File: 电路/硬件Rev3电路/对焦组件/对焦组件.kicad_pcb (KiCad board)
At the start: 2 copper layers, 1 part, among them U1 CH32V003FxPx

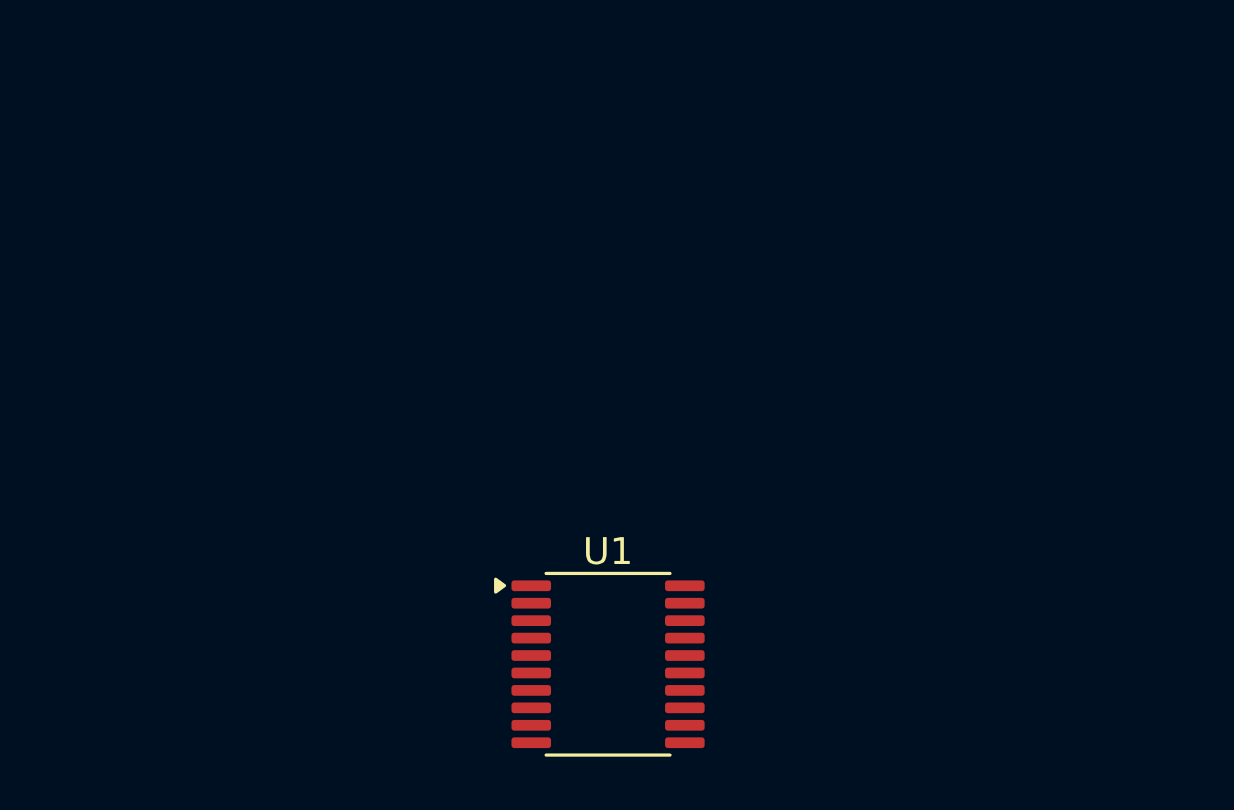
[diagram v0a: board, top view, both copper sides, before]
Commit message: 对焦驱动几乎完成
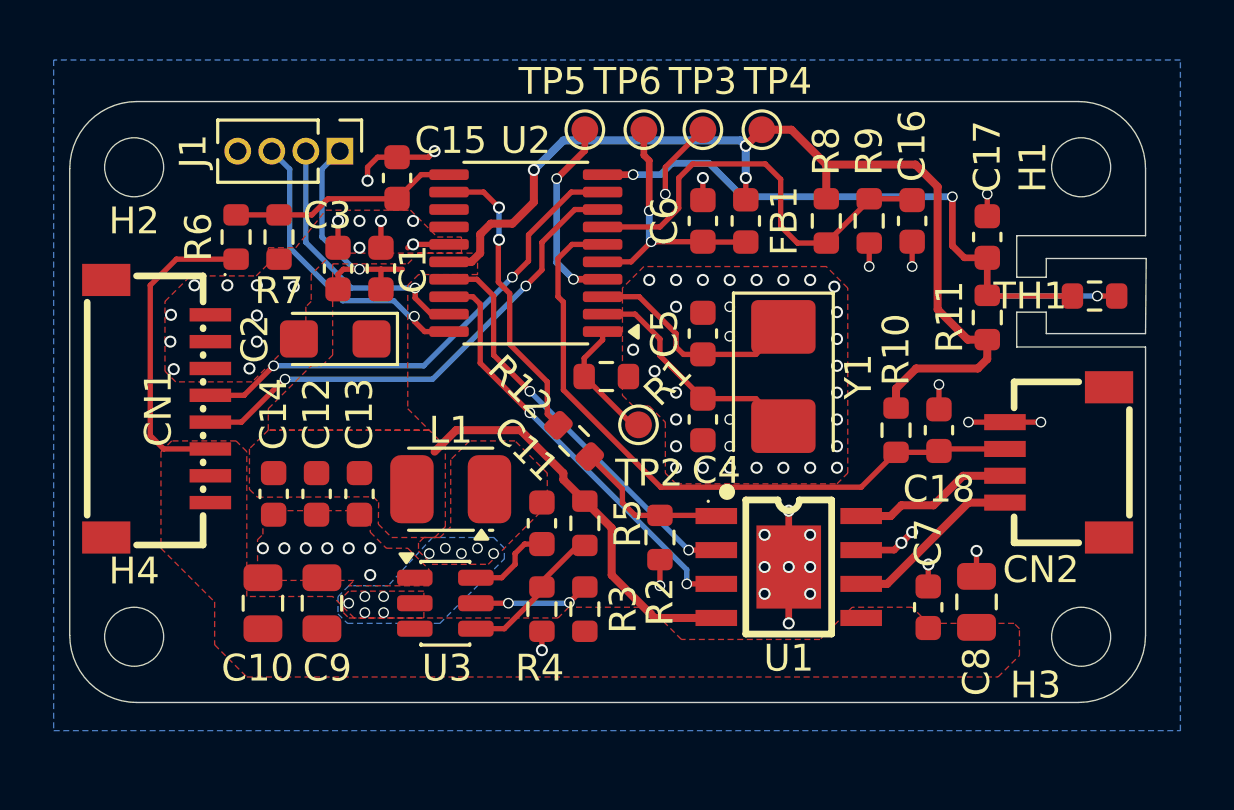
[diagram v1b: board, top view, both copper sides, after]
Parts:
- added C1: 100nf, Capacitor_SMD:C_0603_1608Metric, F.Cu at (109.3, 86.4)
- added C10: 10uf, Capacitor_SMD:C_0805_2012Metric, F.Cu at (104.9, 98.9)
- added C11: 100nf, Capacitor_SMD:C_0603_1608Metric, F.Cu at (115.3, 95.9)
- added C12: 22uf, Capacitor_SMD:C_0603_1608Metric, F.Cu at (106.9, 94.8)
- added C13: 22uf, Capacitor_SMD:C_0603_1608Metric, F.Cu at (108.5, 94.8)
- added C14: 22uf, Capacitor_SMD:C_0603_1608Metric, F.Cu at (105.3, 94.8)
- added C15: 22uf, Capacitor_SMD:C_0603_1608Metric, F.Cu at (109.9, 83.0)
- added C16: 22uf, Capacitor_SMD:C_0603_1608Metric, F.Cu at (129.1, 84.6)
- added C17: 22uf, Capacitor_SMD:C_0603_1608Metric, F.Cu at (131.9, 85.2)
- added C18: 22uf, Capacitor_SMD:C_0603_1608Metric, F.Cu at (130.1, 92.4)
- added C2: 22uf, Capacitor_Tantalum_SMD:CP_EIA-3216-18_Kemet-A, F.Cu at (107.6, 89.0)
- added C3: 1uf, Capacitor_SMD:C_0603_1608Metric, F.Cu at (107.7, 86.4)
- added C4: 20pf, Capacitor_SMD:C_0603_1608Metric, F.Cu at (121.3, 92.0)
- added C5: 20pf, Capacitor_SMD:C_0603_1608Metric, F.Cu at (121.3, 88.8)
- added C6: 100nf, Capacitor_SMD:C_0603_1608Metric, F.Cu at (121.3, 84.6)
- added C7: 100nf, Capacitor_SMD:C_0603_1608Metric, F.Cu at (129.7, 99.0)
- added C8: 47uf, Capacitor_SMD:C_0805_2012Metric, F.Cu at (131.5, 98.8)
- added C9: 10uf, Capacitor_SMD:C_0805_2012Metric, F.Cu at (107.1, 98.9)
- added CN1: HX SH-1.0-8PWT, EasyEDA:CONN-SMD_8P-P1.00_HX-SH1.0-8PWT, F.Cu at (101.0, 91.6)
- added CN2: HX SH-1.0-4PWT, EasyEDA:CONN-SMD_4P-HX-SH-1.0-4PWT, F.Cu at (134.5, 93.6)
- added FB1: FerriteBead, Inductor_SMD:L_0603_1608Metric, F.Cu at (122.9, 84.6)
- added H1: MountingHole, MountingHole:MountingHole_2.2mm_M2, F.Cu at (135.4, 82.6)
- added H2: MountingHole, MountingHole:MountingHole_2.2mm_M2, F.Cu at (100.1, 82.6)
- added H3: MountingHole, MountingHole:MountingHole_2.2mm_M2, F.Cu at (135.4, 100.1)
- added H4: MountingHole, MountingHole:MountingHole_2.2mm_M2, F.Cu at (100.1, 100.1)
- added J1: Conn_01x04_Pin, Connector_PinHeader_1.27mm:PinHeader_1x04_P1.27mm_Vertical, F.Cu at (107.8, 82.0)
- added L1: 2.2uH, Inductor_SMD:L_Coilcraft_1008HQ_2520Metric, F.Cu at (111.9, 94.6)
- added R1: 10k, Resistor_SMD:R_0603_1608Metric, F.Cu at (117.7, 90.4)
- added R10: 10k 1%, Resistor_SMD:R_0603_1608Metric, F.Cu at (128.5, 92.4)
- added R11: 10k 1%, Resistor_SMD:R_0603_1608Metric, F.Cu at (131.9, 88.2)
- added R12: 1k, Resistor_SMD:R_0603_1608Metric, F.Cu at (116.5, 92.8)
- added R2: 10k, Resistor_SMD:R_0603_1608Metric, F.Cu at (119.7, 96.4)
- added R3: 10k, Resistor_SMD:R_0603_1608Metric, F.Cu at (116.9, 99.1)
- added R4: 10k, Resistor_SMD:R_0603_1608Metric, F.Cu at (115.3, 99.1)
- added R5: 33.2k, Resistor_SMD:R_0603_1608Metric, F.Cu at (116.9, 95.9)
- added R6: 10k 1%, Resistor_SMD:R_0603_1608Metric, F.Cu at (103.9, 85.2)
- added R7: 10k 1%, Resistor_SMD:R_0603_1608Metric, F.Cu at (105.5, 85.2)
- added R8: 2.2k 1%, Resistor_SMD:R_0603_1608Metric, F.Cu at (125.9, 84.6)
- added R9: 10k 1%, Resistor_SMD:R_0603_1608Metric, F.Cu at (127.5, 84.6)
- added TH1: Thermistor_NTC, Resistor_SMD:R_0603_1608Metric, F.Cu at (135.9, 87.4)
- added TP2: BOOT, TestPoint:TestPoint_Pad_D1.0mm, F.Cu at (118.9, 92.2)
- added TP3: GND, TestPoint:TestPoint_Pad_D1.0mm, F.Cu at (121.3, 81.2)
- added TP4: 3.3V, TestPoint:TestPoint_Pad_D1.0mm, F.Cu at (123.5, 81.2)
- added TP5: NRST, TestPoint:TestPoint_Pad_D1.0mm, F.Cu at (116.9, 81.2)
- added TP6: VREF, TestPoint:TestPoint_Pad_D1.0mm, F.Cu at (119.1, 81.2)
- added U2: STM32F030F4Px, Package_SO:TSSOP-20_4.4x6.5mm_P0.65mm, F.Cu at (114.7, 85.8)
- added U3: TPS563201, Package_TO_SOT_SMD:SOT-23-6, F.Cu at (111.7, 98.9)
- added Y1: 8Mhz, Crystal:Crystal_SMD_5032-2Pin_5.0x3.2mm, F.Cu at (124.3, 90.4)
- U1: value CH32V003FxPx -> DRV8251ADDAR; footprint Package_SO:TSSOP-20_4.4x6.5mm_P0.65mm -> EasyEDA:SOPOWERPAD-8_L4.9-W3.9-P1.27-LS6.0-TL-EP
- moved U1 7.65 mm to (124.5, 97.5)
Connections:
- U1 pad 1: unconnected-(U1-PD4-Pad1) -> Net-(U1-IPROPI)
- U1 pad 2: unconnected-(U1-PD5-Pad2) -> /MotorPWM_B
- U1 pad 3: unconnected-(U1-PD6-Pad3) -> /MotorPWM_A
- U1 pad 4: unconnected-(U1-PD7-Pad4) -> +3V3
- U1 pad 5: unconnected-(U1-PA1-Pad5) -> +6V
- U1 pad 6: unconnected-(U1-PA2-Pad6) -> /MOT_A
- U1 pad 7: unconnected-(U1-VSS-Pad7) -> GND
- U1 pad 8: unconnected-(U1-PD0-Pad8) -> /MOT_B
- U1 pad 9: unconnected-(U1-VDD-Pad9) -> GND
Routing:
- net +3V3: track 0.00 -> 62.0 mm, vias 0 -> 4
- net GND: track 0.00 -> 31.5 mm, vias 0 -> 80
- net /ADC_NTC1: track 0.00 -> 25.4 mm
- net /ADC_NTC2: track 0.00 -> 21.9 mm, vias 0 -> 2
- net /USART1 _TX: track 0.00 -> 18.6 mm, vias 0 -> 2
- net /USART1 _RX: track 0.00 -> 18.4 mm, vias 0 -> 2
- net /ADC_3V3: track 0.00 -> 16.3 mm
- net /MotorPWM_A: track 0.00 -> 16.0 mm, vias 0 -> 2
- net /MotorPWM_B: track 0.00 -> 15.4 mm, vias 0 -> 2
- net +6V: track 0.00 -> 11.6 mm
- net /SWCLK: track 0.00 -> 11.2 mm, vias 0 -> 1
- net /ADC_MT: track 0.00 -> 11.2 mm, vias 0 -> 2
- net /SWDIO: track 0.00 -> 10.1 mm, vias 0 -> 1
- net Net-(U2-VDDA): track 0.00 -> 9.94 mm, vias 0 -> 2
- net Net-(U2-PF0): track 0.00 -> 8.83 mm
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- added copper zone on F.Cu, net +3V3
- added copper zone on F.Cu, net +6V
- added copper zone on B.Cu, net GND
- added copper zone on F.Cu, net GND
- added copper zone on B.Cu, net Net-(U3-SW)
- added copper zone on F.Cu, net Net-(U3-SW)
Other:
- board outline added: 40.1 x 22.4 mm
